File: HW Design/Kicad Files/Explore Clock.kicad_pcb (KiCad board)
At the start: 2 copper layers, 75 x 45 mm, 29 parts, among them CON1 BARREL_JACK, IC1 ATMEGA328P-P, P1 CONN_01X07, Q1 BC547, Q2 BC547, Q3 IRF540N, SW1 SW_PUSH, SW2 SW_PUSH, U1 LDR, U2 MountingHole, U3 MountingHole, U4 MountingHole, U5 MountingHole, U6 EE_Logo, Y1 32.768KHz

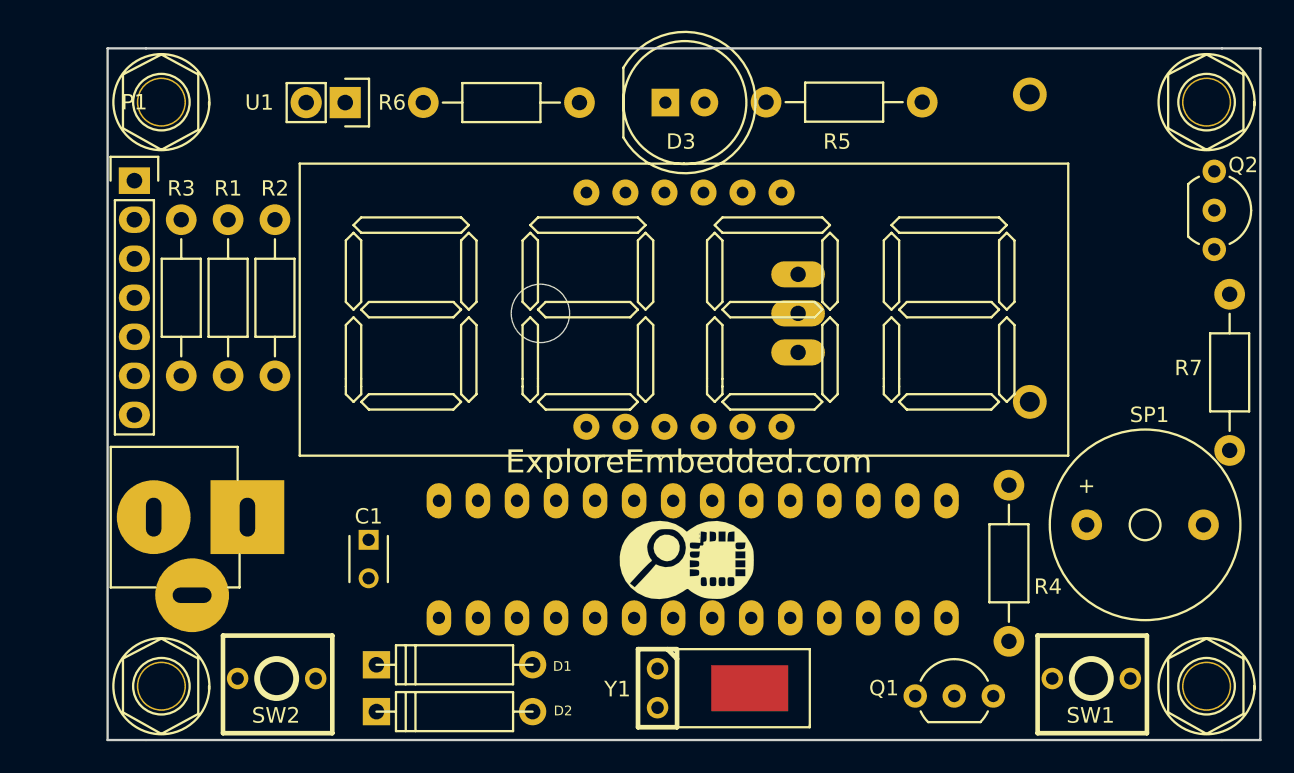
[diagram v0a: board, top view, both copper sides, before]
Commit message: Kicad Design files ready for manufacturing
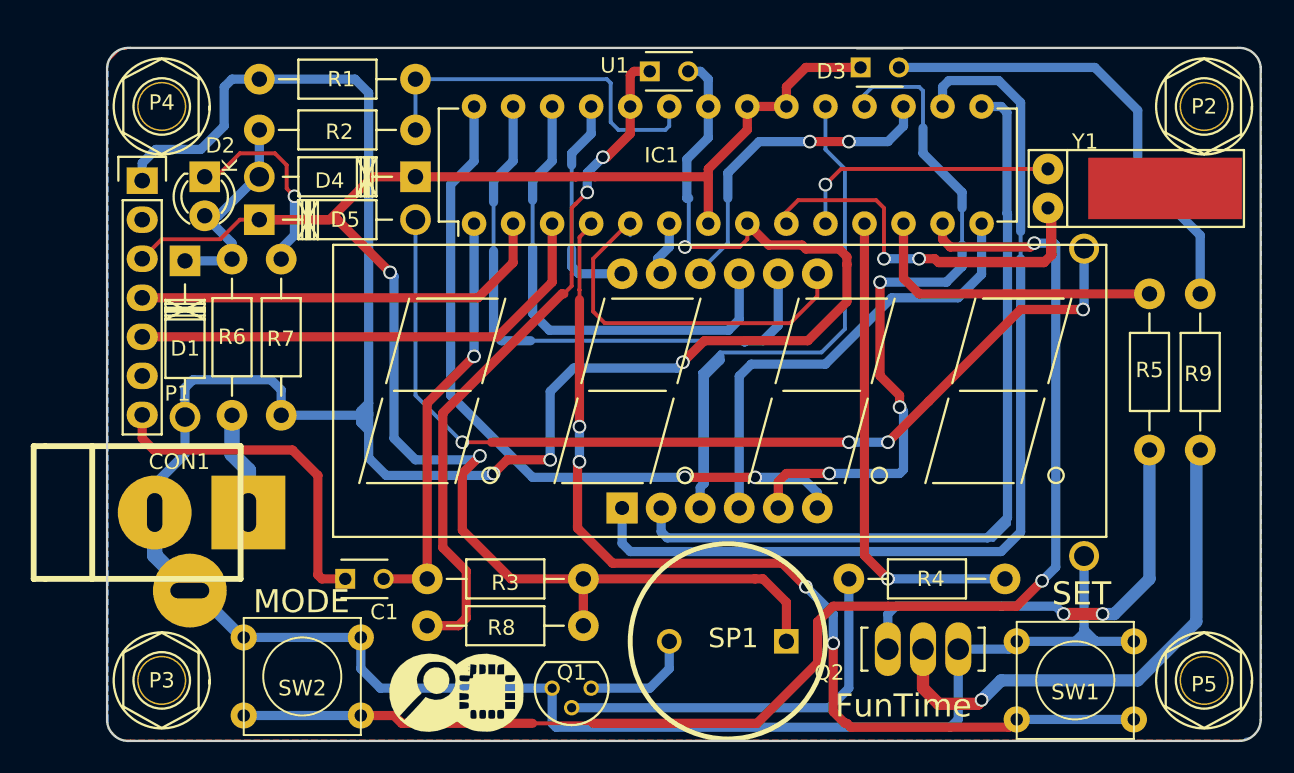
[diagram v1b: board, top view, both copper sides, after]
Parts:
- removed Q3: IRF540N, TO_SOT_Packages_THT:TO-220_Neutral123_Horizontal_LargePads
- removed U2, U3, U4, U5: MountingHole, EE:M3_mounting
- removed U6: EE_Logo, Logo:Logo_8
- added D4: 4148, Diodes_ThroughHole:Diode_DO-41_SOD81_Horizontal_RM10, F.Cu at (192.5, 38.4)
- added D5: 4148, Diodes_ThroughHole:Diode_DO-41_SOD81_Horizontal_RM10, F.Cu at (182.4, 41.1)
- added G***: LOGO, warning Logo:Logo_silk_warning_5x4.2mm, B.Cu at (219.5, 72.1)
- added P14: CONN_01X01, EE:Logo_8, F.Cu at (195.1, 71.9)
- added P14: CONN_01X01, EE:Logo_8, B.Cu at (223.8, 37.3)
- added P2: CONN_01X01, EE:M3_mounting, F.Cu at (243.8, 33.8)
- added P3: CONN_01X01, EE:M3_mounting, F.Cu at (176.0, 71.1)
- added P4: CONN_01X01, EE:M3_mounting, F.Cu at (176.0, 33.8)
- added P5: CONN_01X01, EE:M3_mounting, F.Cu at (243.8, 71.1)
- added R8: 10K, Resistors_ThroughHole:Resistor_Horizontal_RM10mm, F.Cu at (198.4, 67.6)
- added R9: 47E, Resistors_ThroughHole:Resistor_Horizontal_RM10mm, F.Cu at (243.6, 51.1)
- AFF1: footprint EE:4Digit Numeric Display .56inch -> Displays_7-Segment:Cx56-12
- BT1: footprint EE:RTC_Battery_Holder -> EE:BATT_rtc_XL
- CON1: footprint EE:DC_Jack -> EE:JACK_ALIM
- D1: value D_Schottky -> ZENER; footprint EE:Diode_D4 -> Diodes_ThroughHole:Diode_DO-41_SOD81_Horizontal_RM10
- D2: value D_Schottky -> PLED; footprint EE:Diode_D4 -> LEDs:LED-3MM
- D3: footprint LEDs:LED-8MM -> Capacitors_ThroughHole:C_Disc_D3_P2.5
- IC1: footprint Housings_DIP:DIP-28_W7.62mm_LongPads -> Housings_DIP:DIP-28_W7.62mm; moved to F.Cu
- Q1: footprint TO_SOT_Packages_THT:TO-92_Inline_Wide -> TO_SOT_Packages_THT:TO-92_Molded_Narrow
- Q2: value BC547 -> BD139; footprint TO_SOT_Packages_THT:TO-92_Inline_Wide -> TO_SOT_Packages_THT:SOT126_SOT32_Housing_Vertical_BigPads
- R1: value E -> 100K
- R2: value E -> 10K
- R6: value 100K -> 1K
- R7: value 5E/1W -> 1K
- SP1: footprint Buzzers_Beepers:Buzzer_12x9.5RM7.6 -> EE:BUZ3-5
- SW1, SW2: footprint EE:SW_PUSH_SMALL_2pin_3D_xl_v1 -> EE:SW_PUSH_SMALL
- U1: footprint Pin_Headers:Pin_Header_Straight_1x02 -> Capacitors_ThroughHole:C_Disc_D3_P2.5
- Y1: footprint EE:RTC_Crystal_1 -> EE:RTC_Crystal
- moved R7 62.2 mm to (183.8, 53.9), turned to 90 degrees
- moved Y1 41.3 mm to (233.7, 39.1)
- moved IC1 40.0 mm to (196.3, 41.4)
- moved D2 38.4 mm to (178.8, 38.4), turned to 270 degrees
- moved Q2 36.4 mm to (225.6, 69.1), turned to 180 degrees
- moved R3 35.1 mm to (203.5, 64.5), turned to 180 degrees
- moved D1 31.6 mm to (177.5, 43.8), turned to 270 degrees
- moved R6 30.4 mm to (180.6, 53.9), turned to 90 degrees
- moved SP1 28.2 mm to (212.9, 68.6), turned to 180 degrees
- moved R5 27.0 mm to (240.3, 56.1), turned to 90 degrees
- moved Q1 21.1 mm to (204.0, 71.6), turned to 180 degrees
- moved U1 19.9 mm to (207.8, 31.5), turned to 0 degrees
- moved R2 16.0 mm to (182.4, 35.3), turned to 0 degrees
- moved R1 15.2 mm to (192.5, 32.0), turned to 180 degrees
- moved AFF1 13.5 mm to (206.0, 59.9)
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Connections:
- D1 pad 1: VCC -> Net-(D1-Pad1)
- D1 pad 2: Net-(CON1-Pad1) -> GND
- D2 pad 1: VCC -> Net-(D2-Pad1)
- D2 pad 2: Net-(BT1-Pad1) -> Net-(D1-Pad1)
- IC1 pad 4: /A -> /SET
- IC1 pad 6: /SET -> /A
- Q2 pad 1: Net-(Q2-Pad1) -> GND
- Q2 pad 3: GND -> Net-(Q2-Pad3)
- R2 pad 1: Net-(CON1-Pad1) -> Net-(D1-Pad1)
- R5 pad 1: Net-(Q2-Pad1) -> Net-(Q2-Pad3)
- R6 pad 1: VCC -> Net-(CON1-Pad1)
- R6 pad 2: Net-(IC1-Pad24) -> Net-(D1-Pad1)
- R7 pad 1: Net-(Q2-Pad2) -> GND
- R7 pad 2: GND -> Net-(D2-Pad1)
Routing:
- net GND: track 0.00 -> 317.7 mm, vias 0 -> 4
- net VCC: track 0.00 -> 161.6 mm, vias 0 -> 2
- net /Mode: track 0.00 -> 150.4 mm, vias 0 -> 2
- net /D: track 0.00 -> 105.2 mm
- net /SET: track 0.00 -> 97.1 mm, vias 0 -> 4
- net /E: track 0.00 -> 90.8 mm
- net /Digit4: track 0.00 -> 76.3 mm, vias 0 -> 2
- net /G: track 0.00 -> 69.1 mm, vias 0 -> 3
- net Net-(BT1-Pad1): track 0.00 -> 67.8 mm, vias 0 -> 4
- net Net-(IC1-Pad24): track 0.00 -> 65.1 mm, vias 0 -> 2
- net Net-(Q2-Pad2): track 0.00 -> 60.2 mm, vias 0 -> 1
- net /C: track 0.00 -> 57.5 mm
- net /TXD: track 0.00 -> 52.7 mm
- net Net-(Q2-Pad3): track 0.00 -> 52.5 mm, vias 0 -> 2
- net Net-(D3-Pad2): track 0.00 -> 47.9 mm
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- added copper zone on B.Cu, net GND
- added copper zone on F.Cu, net VCC
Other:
- board size 75 x 45 mm -> 75.1 x 45.1 mm
- board text added: "FunTime"
- board text added: "MODE"
- board text added: "MODE : Switch between Time , Alarm and Light control. SET : Set the values for modes."
- board text added: "SET"
- board text added: "Use +5V DC adapter only"
